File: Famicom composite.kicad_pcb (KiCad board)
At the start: 2 copper layers, 14.2 x 19.9 mm, 11 parts, among them J1 PPU_Pin21, J2 Conn_01x02, J3 Audio_In, J4 Conn_01x04_Female, U1 THS7314

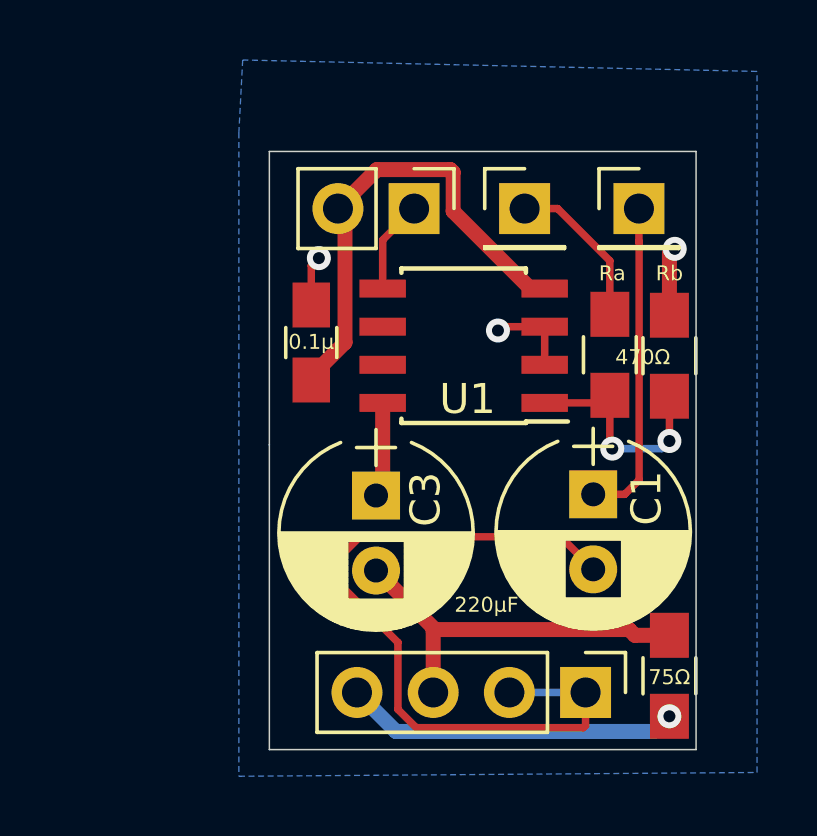
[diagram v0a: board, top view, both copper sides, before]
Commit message: BBCBC version sent to Osh
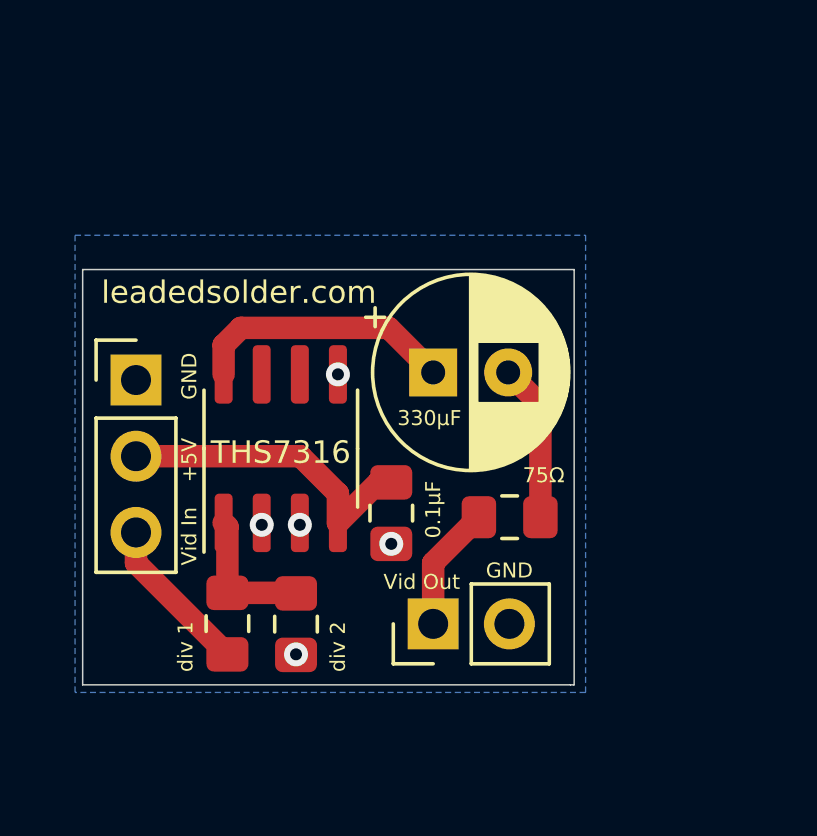
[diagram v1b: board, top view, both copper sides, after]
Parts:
- removed C1: 220µF, Capacitors_ThroughHole:CP_Radial_D6.3mm_P2.50mm
- removed J2: Conn_01x02, Pin_Headers:Pin_Header_Straight_1x02_Pitch2.54mm
- removed J4: Conn_01x04_Female, Pin_Headers:Pin_Header_Straight_1x04_Pitch2.54mm
- C2: footprint Capacitors_SMD:C_0805_HandSoldering -> Capacitor_SMD:C_0805_2012Metric_Pad1.15x1.40mm_HandSolder
- C3: footprint Capacitors_ThroughHole:CP_Radial_D6.3mm_P2.50mm -> Capacitor_THT:CP_Radial_D6.3mm_P2.50mm
- J1: value PPU_Pin21 -> Conn_01x03_Female; footprint Pin_Headers:Pin_Header_Straight_1x01_Pitch2.54mm -> Connector_PinHeader_2.54mm:PinHeader_1x03_P2.54mm_Vertical
- J3: value Audio_In -> Conn_01x02_Female; footprint Pin_Headers:Pin_Header_Straight_1x01_Pitch2.54mm -> Connector_PinHeader_2.54mm:PinHeader_1x02_P2.54mm_Vertical
- R1: value 470Ω -> 1500Ω; footprint Resistors_SMD:R_0805_HandSoldering -> Resistor_SMD:R_0805_2012Metric_Pad1.15x1.40mm_HandSolder
- R2, R3: footprint Resistors_SMD:R_0805_HandSoldering -> Resistor_SMD:R_0805_2012Metric_Pad1.15x1.40mm_HandSolder
- U1: footprint Housings_SOIC:SOIC-8_3.9x4.9mm_Pitch1.27mm -> Package_SO:SOIC-8_3.9x4.9mm_P1.27mm
- moved R1 15.6 mm to (126.7, 102.1), turned to 90 degrees
- moved J3 15.4 mm to (133.6, 102.1), turned to 90 degrees
- moved R3 15.3 mm to (129.0, 102.1), turned to 270 degrees
- moved J1 14.2 mm to (123.7, 94.0)
- moved R2 7.50 mm to (136.2, 98.6), turned to 180 degrees
- moved U1 6.99 mm to (128.5, 96.3), turned to 90 degrees
- moved C2 6.28 mm to (132.2, 98.4), turned to 270 degrees
- moved C3 4.52 mm to (133.6, 93.7), turned to 0 degrees
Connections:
- net /Half_Vpp renamed /Chopped_Vpp
- C3 pad 2: /Vid_Out -> Net-(C3-Pad2)
- J1 pad 1: Net-(J1-Pad1) -> GND
- J3 pad 1: Net-(C1-Pad1) -> /Vid_Out
- R1 pad 1: Net-(J1-Pad1) -> /Pre_RF
- R2 pad 1: GND -> Net-(C3-Pad2)
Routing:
- net Net-(C1-Pad2): track 25.2 -> 0.00 mm
- net GND: track 21.1 -> 0.00 mm, vias 4 -> 5
- net Net-(C1-Pad1): track 10.8 -> 0.00 mm
- net /Vid_Out: track 12.8 -> 4.19 mm
- net Net-(C3-Pad1): track 3.18 -> 8.81 mm
- net +5V: track 16.1 -> 10.6 mm
- net Net-(J1-Pad1): track 5.34 -> 0.00 mm
- net /Pre_RF: track 0.00 -> 5.33 mm
- net Net-(C3-Pad2): track 0.00 -> 5.27 mm
- net /Chopped_Vpp: track 7.59 -> 4.68 mm, vias 2 -> 0
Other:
- board size 14.2 x 19.9 mm -> 16.4 x 13.8 mm
- board text added: "+5V"
- board text added: "0.1µF"
- board text added: "330µF"
- board text added: "THS7316"
- board text added: "Vid In"
- board text added: "Vid Out"
- board text added: "bbc bridge composite mod v0.1"
- board text added: "div 1"
- board text added: "div 2"
- board text added: "leadedsolder.com"
- board text removed: "0.1µ"
- board text removed: "220µF"
- board text removed: "470Ω"
- board text removed: "5V"
- board text removed: "Aud In"
- board text removed: "Audio Out"
- board text removed: "PPU pin21"
- board text removed: "Ra"
- board text removed: "Rb"
- board text removed: "Vid"
- board text removed: "fami composite board v0.6"
- board text removed: "leadedsolder.com 2020"
